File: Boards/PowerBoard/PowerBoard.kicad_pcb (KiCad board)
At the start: 4 copper layers, 430 x 310 mm, 224 parts, among them IC10 ACS772ECB-400B-PFF-T, IC3 ACS772ECB-400B-PFF-T, IC4 ACS772ECB-400B-PFF-T, IC5 ACS772ECB-400B-PFF-T, IC6 ACS772ECB-400B-PFF-T, IC7 ACS772ECB-400B-PFF-T, IC8 ACS772ECB-400B-PFF-T, IC9 ACS772ECB-400B-PFF-T, J6 L717SDB25PA4CH3R, J8 Conn_01x10_Socket, J9 Conn_01x10_Socket

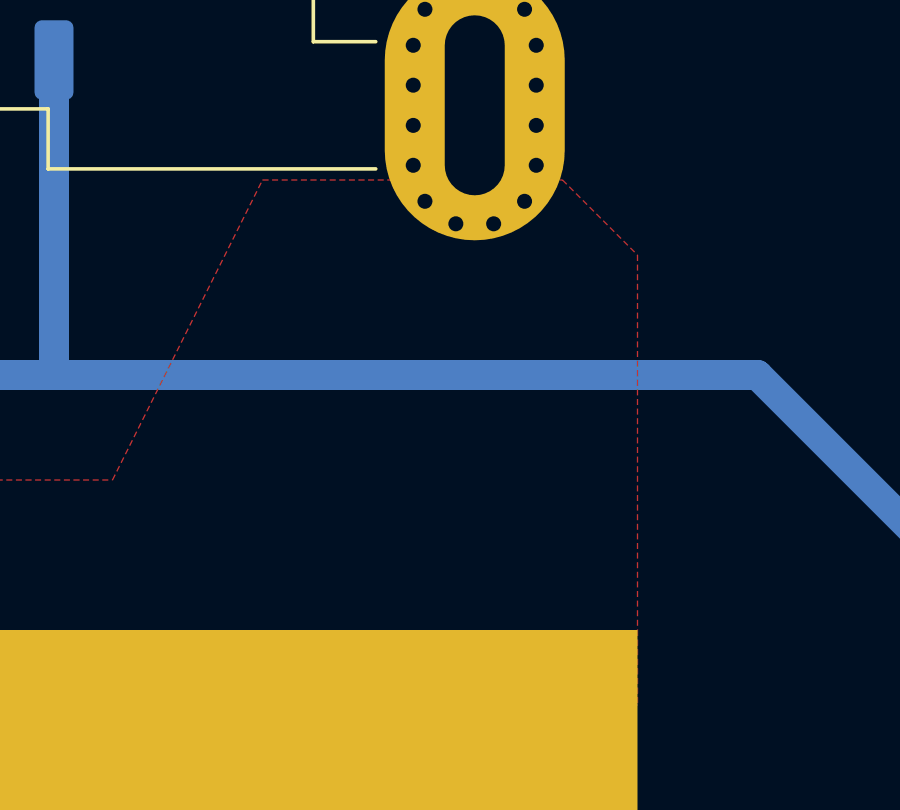
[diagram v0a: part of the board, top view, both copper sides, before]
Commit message: Update Layouts
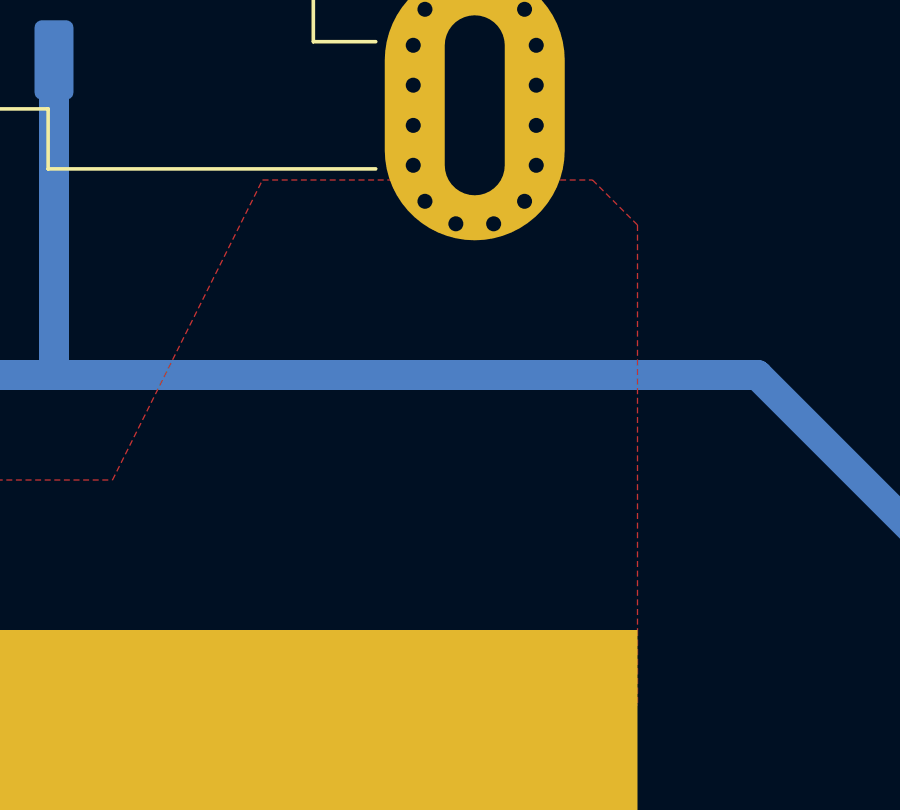
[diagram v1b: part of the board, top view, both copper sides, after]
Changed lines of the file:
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@@
 	(gr_poly
 		(pts
-			(xy -81.5 17.5) (xy -76.5 13) (xy 277 13) (xy 277 30) (xy -52 30) (xy -52 30) (xy -81.5 30)
+			(xy -81.5 17.5) (xy -76.5 13) (xy 277 13) (xy 277 30) (xy -52 30) (xy -81.5 30)
 		)
 		(stroke
@@
 		(layer "F.Mask")
 	)
+	(gr_rect
+		(start -82 45)
+		(end -73 60)
+		(stroke
+			(width 0.1)
+			(type solid)
+		)
+		(fill yes)
+		(layer "F.Mask")
+	)
+	(gr_rect
+		(start -48.5 45)
+		(end -39.5 60)
+		(stroke
+			(width 0.1)
+			(type solid)
+		)
+		(fill yes)
+		(layer "F.Mask")
+	)
 	(gr_poly
 		(pts
@@
 		(polygon
 			(pts
-				(xy -85 47.5) (xy -82.5 45) (xy -72.5 45) (xy -67.5 55) (xy -55 55) (xy -50 45) (xy -40 45) (xy -37.5 47.5)
+				(xy -85 47.5) (xy -82.5 45) (xy -72.5 45) (xy -67.5 55) (xy -55 55) (xy -50 45) (xy -39 45) (xy -37.5 46.5)
 				(xy -37.5 60) (xy -37.5 62.5) (xy -87.5 62.5) (xy -87.5 60) (xy -85 57.5)
 			)
